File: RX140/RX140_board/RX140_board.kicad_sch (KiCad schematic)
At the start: 1 part

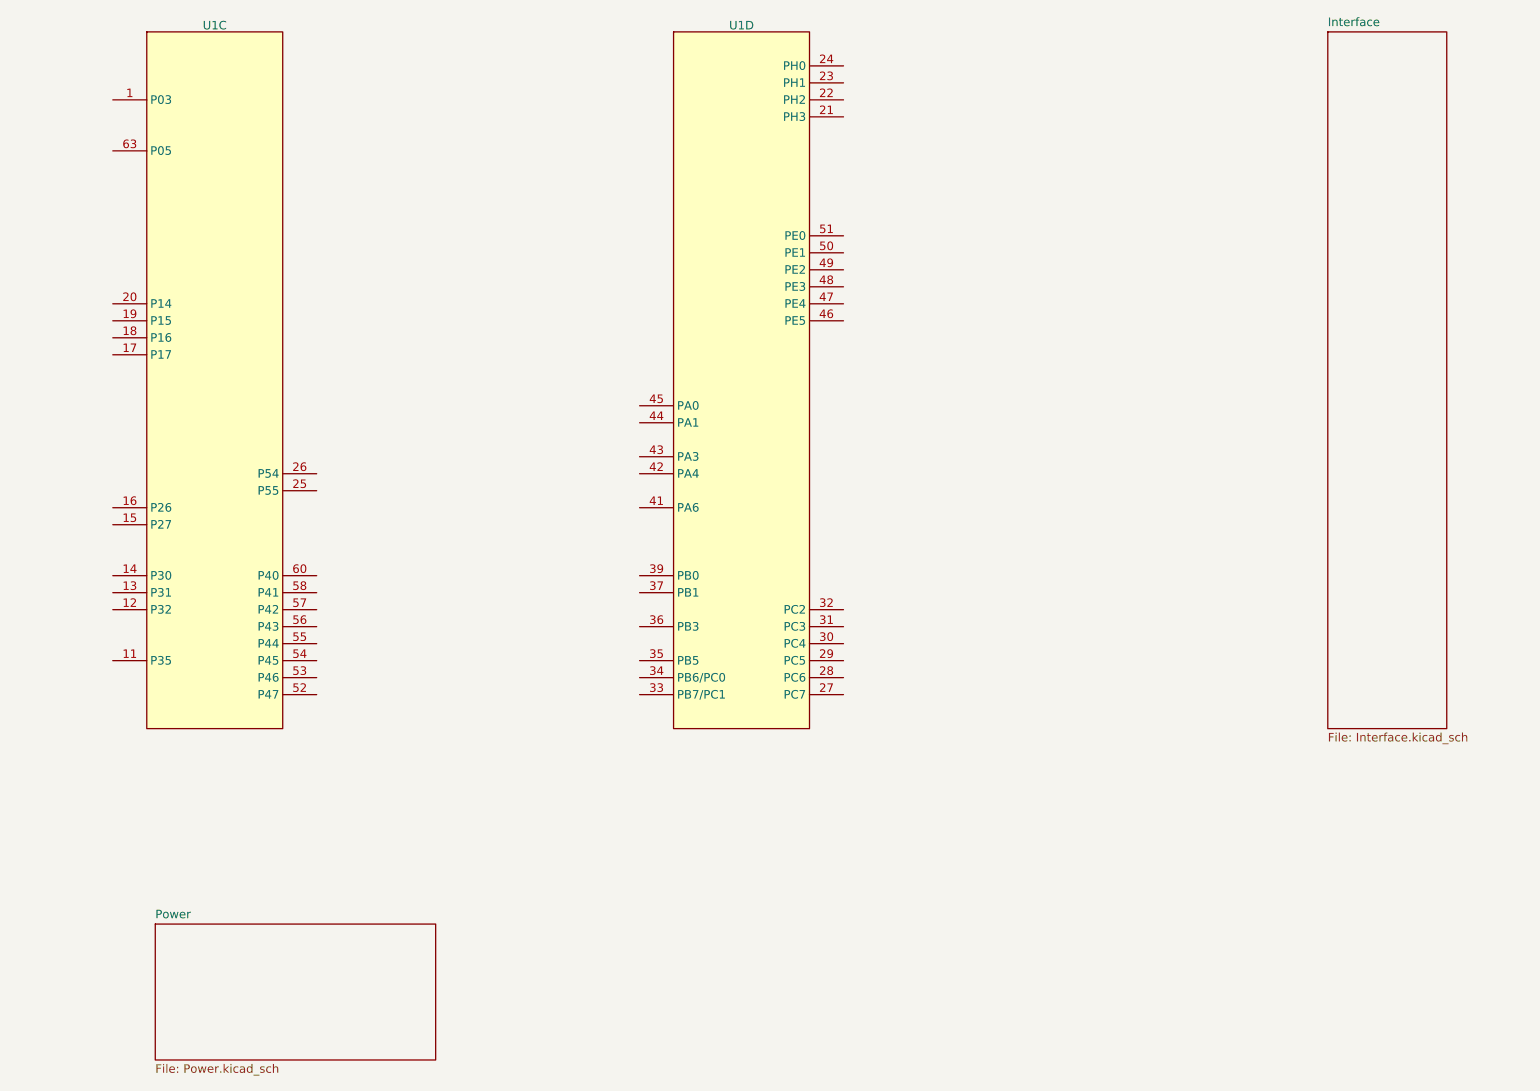
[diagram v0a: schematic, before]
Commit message: Update: cleanup
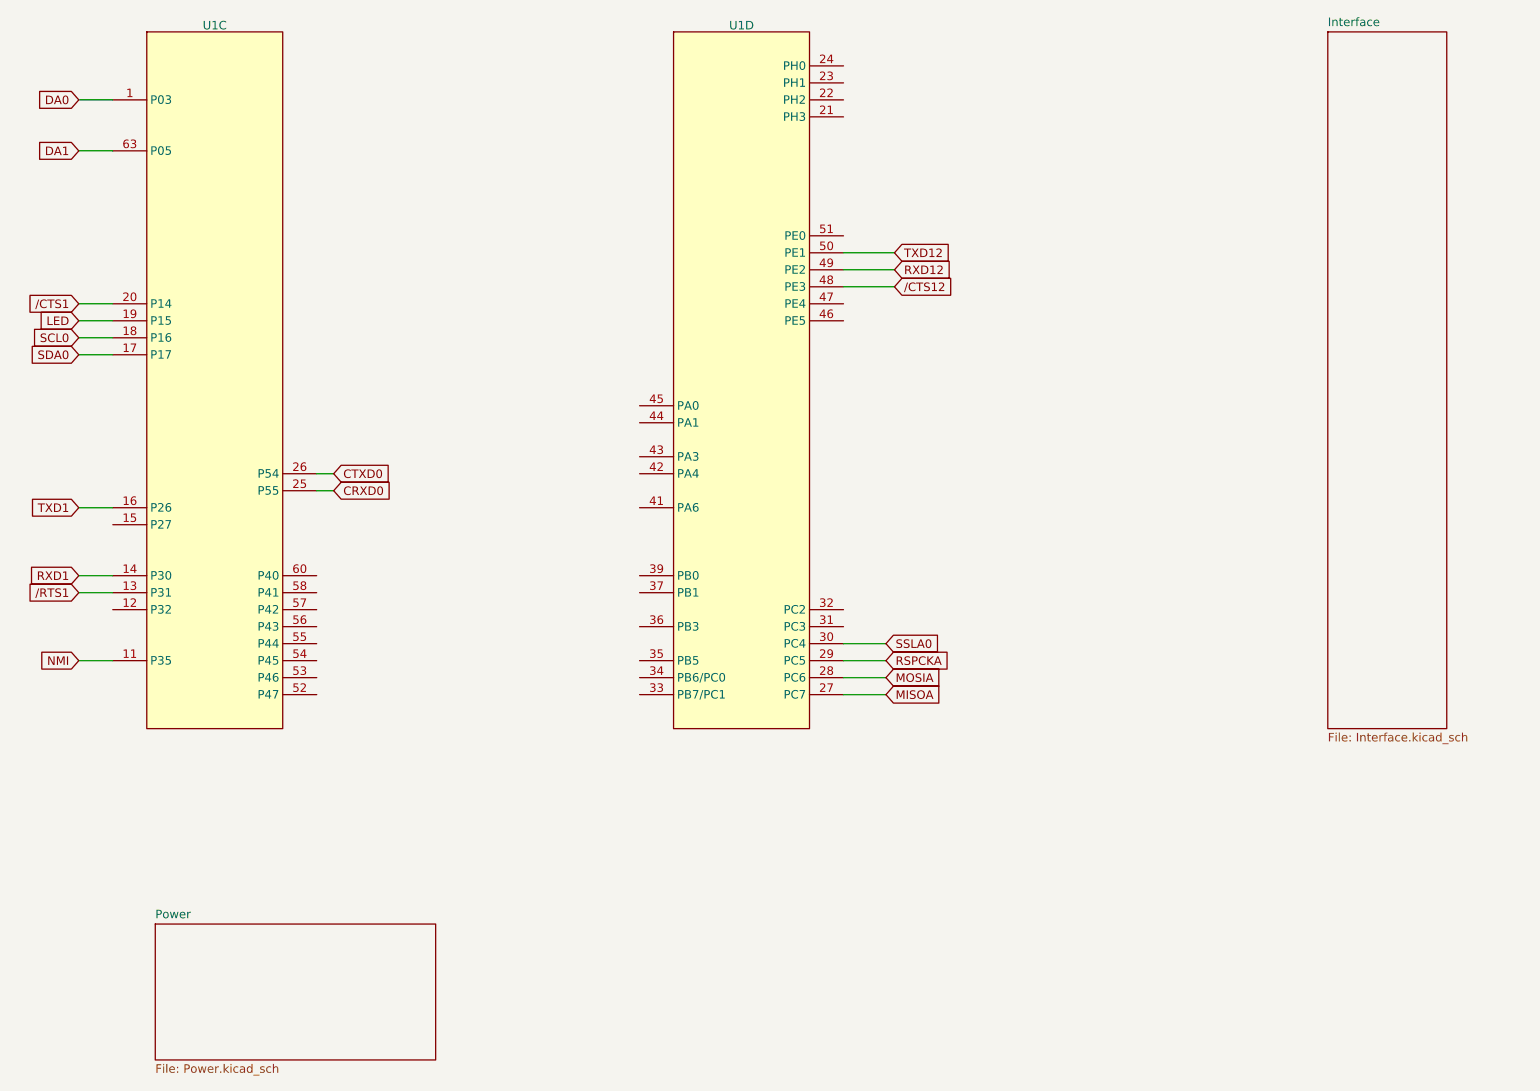
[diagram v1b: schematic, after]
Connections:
- net DA0: now reaches U1.1 (P03)
- net NMI: now reaches U1.11 (P35)
- net /RTS1: now reaches U1.13 (P31)
- net RXD1: now reaches U1.14 (P30)
- net TXD1: now reaches U1.16 (P26)
- net SDA0: now reaches U1.17 (P17)
- net SCL0: now reaches U1.18 (P16)
- net LED: now reaches U1.19 (P15)
- net /CTS1: now reaches U1.20 (P14)
- net CRXD0: now reaches U1.25 (P55)
- net CTXD0: now reaches U1.26 (P54)
- net DA1: now reaches U1.63 (P05)
- net MISOA: now reaches U1.27 (PC7)
- net MOSIA: now reaches U1.28 (PC6)
- net RSPCKA: now reaches U1.29 (PC5)
- net SSLA0: now reaches U1.30 (PC4)
- net /CTS12: now reaches U1.48 (PE3)
- net RXD12: now reaches U1.49 (PE2)
- net TXD12: now reaches U1.50 (PE1)
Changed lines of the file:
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@@
 (kicad_sch (version 20230121) (generator eeschema)
   (paper "A4")
+  (wire (pts (xy 165.1 62.23) (xy 172.72 62.23))
+    (stroke (width 0) (type default))
+  )
+  (wire (pts (xy 50.8 67.31) (xy 55.88 67.31))
+    (stroke (width 0) (type default))
+  )
+  (wire (pts (xy 50.8 64.77) (xy 55.88 64.77))
+    (stroke (width 0) (type default))
+  )
+  (wire (pts (xy 50.8 41.91) (xy 55.88 41.91))
+    (stroke (width 0) (type default))
+  )
+  (wire (pts (xy 165.1 59.69) (xy 172.72 59.69))
+    (stroke (width 0) (type default))
+  )
+  (wire (pts (xy 165.1 118.11) (xy 171.45 118.11))
+    (stroke (width 0) (type default))
+  )
+  (wire (pts (xy 50.8 105.41) (xy 55.88 105.41))
+    (stroke (width 0) (type default))
+  )
+  (wire (pts (xy 165.1 57.15) (xy 172.72 57.15))
+    (stroke (width 0) (type default))
+  )
+  (wire (pts (xy 165.1 120.65) (xy 171.45 120.65))
+    (stroke (width 0) (type default))
+  )
+  (wire (pts (xy 86.36 92.71) (xy 88.9 92.71))
+    (stroke (width 0) (type default))
+  )
+  (wire (pts (xy 86.36 90.17) (xy 88.9 90.17))
+    (stroke (width 0) (type default))
+  )
+  (wire (pts (xy 50.8 72.39) (xy 55.88 72.39))
+    (stroke (width 0) (type default))
+  )
+  (wire (pts (xy 50.8 34.29) (xy 55.88 34.29))
+    (stroke (width 0) (type default))
+  )
+  (wire (pts (xy 50.8 95.25) (xy 55.88 95.25))
+    (stroke (width 0) (type default))
+  )
+  (wire (pts (xy 165.1 115.57) (xy 171.45 115.57))
+    (stroke (width 0) (type default))
+  )
+  (wire (pts (xy 165.1 123.19) (xy 171.45 123.19))
+    (stroke (width 0) (type default))
+  )
+  (wire (pts (xy 50.8 69.85) (xy 55.88 69.85))
+    (stroke (width 0) (type default))
+  )
+  (wire (pts (xy 50.8 107.95) (xy 55.88 107.95))
+    (stroke (width 0) (type default))
+  )
+  (wire (pts (xy 50.8 118.11) (xy 55.88 118.11))
+    (stroke (width 0) (type default))
+  )
+  (global_label "{slash}CTS1" (shape input) (at 50.8 64.77 180) (fields_autoplaced)
+    (effects (font (size 1.27 1.27)) (justify right))
+    (property "Intersheetrefs" "${INTERSHEET_REFS}" (at 41.9071 64.77 0)
+      (effects (font (size 1.27 1.27)) (justify right) hide)
+    )
+  )
+  (global_label "MISOA" (shape input) (at 171.45 123.19 0) (fields_autoplaced)
+    (effects (font (size 1.27 1.27)) (justify left))
+    (property "Intersheetrefs" "${INTERSHEET_REFS}" (at 180.0406 123.19 0)
+      (effects (font (size 1.27 1.27)) (justify left) hide)
+    )
+  )
+  (global_label "DA1" (shape input) (at 50.8 41.91 180) (fields_autoplaced)
+    (effects (font (size 1.27 1.27)) (justify right))
+    (property "Intersheetrefs" "${INTERSHEET_REFS}" (at 44.3261 41.91 0)
+      (effects (font (size 1.27 1.27)) (justify right) hide)
+    )
+  )
+  (global_label "RXD1" (shape input) (at 50.8 105.41 180) (fields_autoplaced)
+    (effects (font (size 1.27 1.27)) (justify right))
+    (property "Intersheetrefs" "${INTERSHEET_REFS}" (at 42.9352 105.41 0)
+      (effects (font (size 1.27 1.27)) (justify right) hide)
+    )
+  )
+  (global_label "LED" (shape input) (at 50.8 67.31 180) (fields_autoplaced)
+    (effects (font (size 1.27 1.27)) (justify right))
+    (property "Intersheetrefs" "${INTERSHEET_REFS}" (at 44.4471 67.31 0)
+      (effects (font (size 1.27 1.27)) (justify right) hide)
+    )
+  )
+  (global_label "CRXD0" (shape input) (at 88.9 92.71 0) (fields_autoplaced)
+    (effects (font (size 1.27 1.27)) (justify left))
+    (property "Intersheetrefs" "${INTERSHEET_REFS}" (at 98.0348 92.71 0)
+      (effects (font (size 1.27 1.27)) (justify left) hide)
+    )
+  )
+  (global_label "TXD12" (shape input) (at 172.72 57.15 0) (fields_autoplaced)
+    (effects (font (size 1.27 1.27)) (justify left))
+    (property "Intersheetrefs" "${INTERSHEET_REFS}" (at 181.4919 57.15 0)
+      (effects (font (size 1.27 1.27)) (justify left) hide)
+    )
+  )
+  (global_label "{slash}RTS1" (shape input) (at 50.8 107.95 180) (fields_autoplaced)
+    (effects (font (size 1.27 1.27)) (justify right))
+    (property "Intersheetrefs" "${INTERSHEET_REFS}" (at 41.9071 107.95 0)
+      (effects (font (size 1.27 1.27)) (justify right) hide)
+    )
+  )
+  (global_label "{slash}CTS12" (shape input) (at 172.72 62.23 0) (fields_autoplaced)
+    (effects (font (size 1.27 1.27)) (justify left))
+    (property "Intersheetrefs" "${INTERSHEET_REFS}" (at 182.8224 62.23 0)
+      (effects (font (size 1.27 1.27)) (justify left) hide)
+    )
+  )
+  (global_label "RXD12" (shape input) (at 172.72 59.69 0) (fields_autoplaced)
+    (effects (font (size 1.27 1.27)) (justify left))
+    (property "Intersheetrefs" "${INTERSHEET_REFS}" (at 181.7943 59.69 0)
+      (effects (font (size 1.27 1.27)) (justify left) hide)
+    )
+  )
+  (global_label "RSPCKA" (shape input) (at 171.45 118.11 0) (fields_autoplaced)
+    (effects (font (size 1.27 1.27)) (justify left))
+    (property "Intersheetrefs" "${INTERSHEET_REFS}" (at 181.7339 118.11 0)
+      (effects (font (size 1.27 1.27)) (justify left) hide)
+    )
+  )
+  (global_label "SSLA0" (shape input) (at 171.45 115.57 0) (fields_autoplaced)
+    (effects (font (size 1.27 1.27)) (justify left))
+    (property "Intersheetrefs" "${INTERSHEET_REFS}" (at 180.101 115.57 0)
+      (effects (font (size 1.27 1.27)) (justify left) hide)
+    )
+  )
+  (global_label "SDA0" (shape input) (at 50.8 72.39 180) (fields_autoplaced)
+    (effects (font (size 1.27 1.27)) (justify right))
+    (property "Intersheetrefs" "${INTERSHEET_REFS}" (at 43.1166 72.39 0)
+      (effects (font (size 1.27 1.27)) (justify right) hide)
+    )
+  )
+  (global_label "TXD1" (shape input) (at 50.8 95.25 180) (fields_autoplaced)
+    (effects (font (size 1.27 1.27)) (justify right))
+    (property "Intersheetrefs" "${INTERSHEET_REFS}" (at 43.2376 95.25 0)
+      (effects (font (size 1.27 1.27)) (justify right) hide)
+    )
+  )
+  (global_label "DA0" (shape input) (at 50.8 34.29 180) (fields_autoplaced)
+    (effects (font (size 1.27 1.27)) (justify right))
+    (property "Intersheetrefs" "${INTERSHEET_REFS}" (at 44.3261 34.29 0)
+      (effects (font (size 1.27 1.27)) (justify right) hide)
+    )
+  )
+  (global_label "SCL0" (shape input) (at 50.8 69.85 180) (fields_autoplaced)
+    (effects (font (size 1.27 1.27)) (justify right))
+    (property "Intersheetrefs" "${INTERSHEET_REFS}" (at 43.1771 69.85 0)
+      (effects (font (size 1.27 1.27)) (justify right) hide)
+    )
+  )
+  (global_label "MOSIA" (shape input) (at 171.45 120.65 0) (fields_autoplaced)
+    (effects (font (size 1.27 1.27)) (justify left))
+    (property "Intersheetrefs" "${INTERSHEET_REFS}" (at 180.0406 120.65 0)
+      (effects (font (size 1.27 1.27)) (justify left) hide)
+    )
+  )
+  (global_label "NMI" (shape input) (at 50.8 118.11 180) (fields_autoplaced)
+    (effects (font (size 1.27 1.27)) (justify right))
+    (property "Intersheetrefs" "${INTERSHEET_REFS}" (at 44.5075 118.11 0)
+      (effects (font (size 1.27 1.27)) (justify right) hide)
+    )
+  )
+  (global_label "CTXD0" (shape input) (at 88.9 90.17 0) (fields_autoplaced)
+    (effects (font (size 1.27 1.27)) (justify left))
+    (property "Intersheetrefs" "${INTERSHEET_REFS}" (at 97.7324 90.17 0)
+      (effects (font (size 1.27 1.27)) (justify left) hide)
+    )
+  )
   (symbol (lib_id "renesas:RX140_64") (at 71.12 76.2 0) (unit 3)
     (in_bom yes) (on_board yes) (dnp no) (fields_autoplaced)
